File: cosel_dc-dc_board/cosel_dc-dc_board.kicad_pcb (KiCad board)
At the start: 2 copper layers, 105 x 80 mm, 15 parts, among them J1 B2PS-VH(LF)(SN), J2 Screw_Terminal_01x02, J3 Screw_Terminal_01x02, U1 CBS

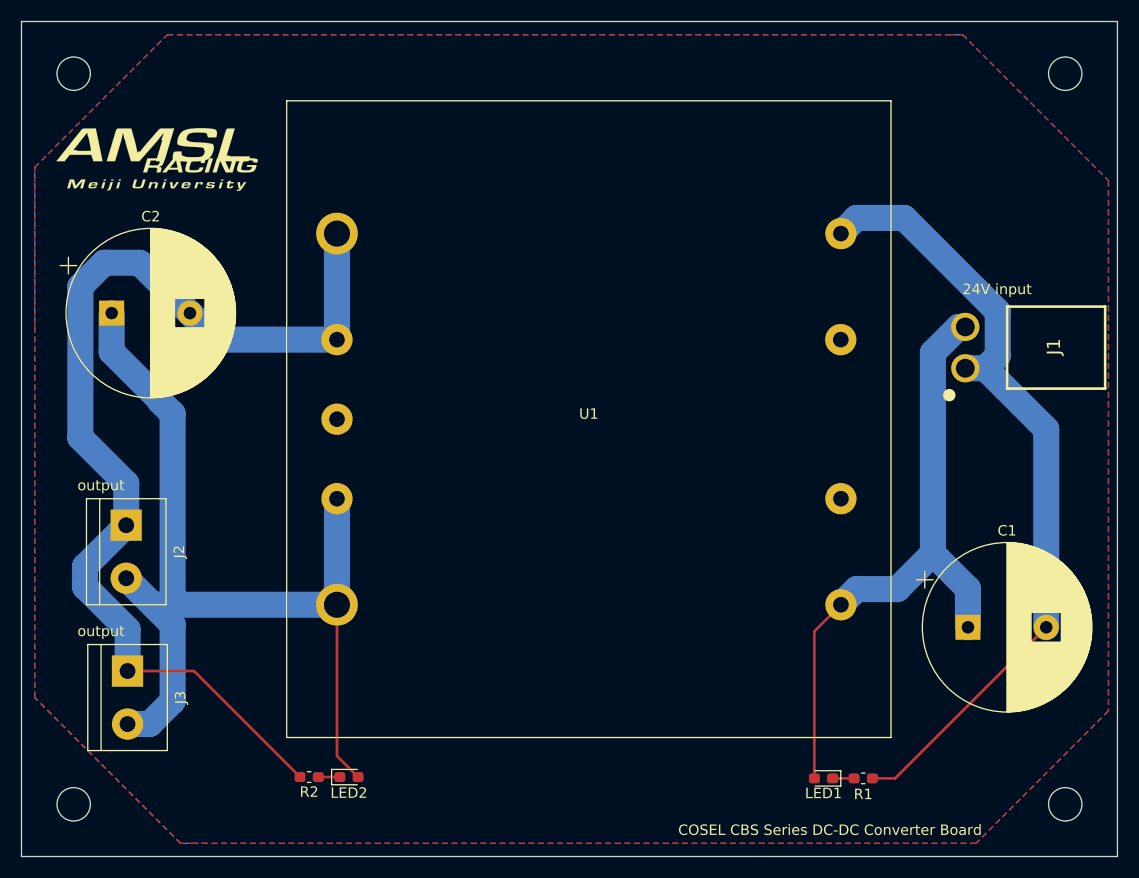
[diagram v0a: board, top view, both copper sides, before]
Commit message: update
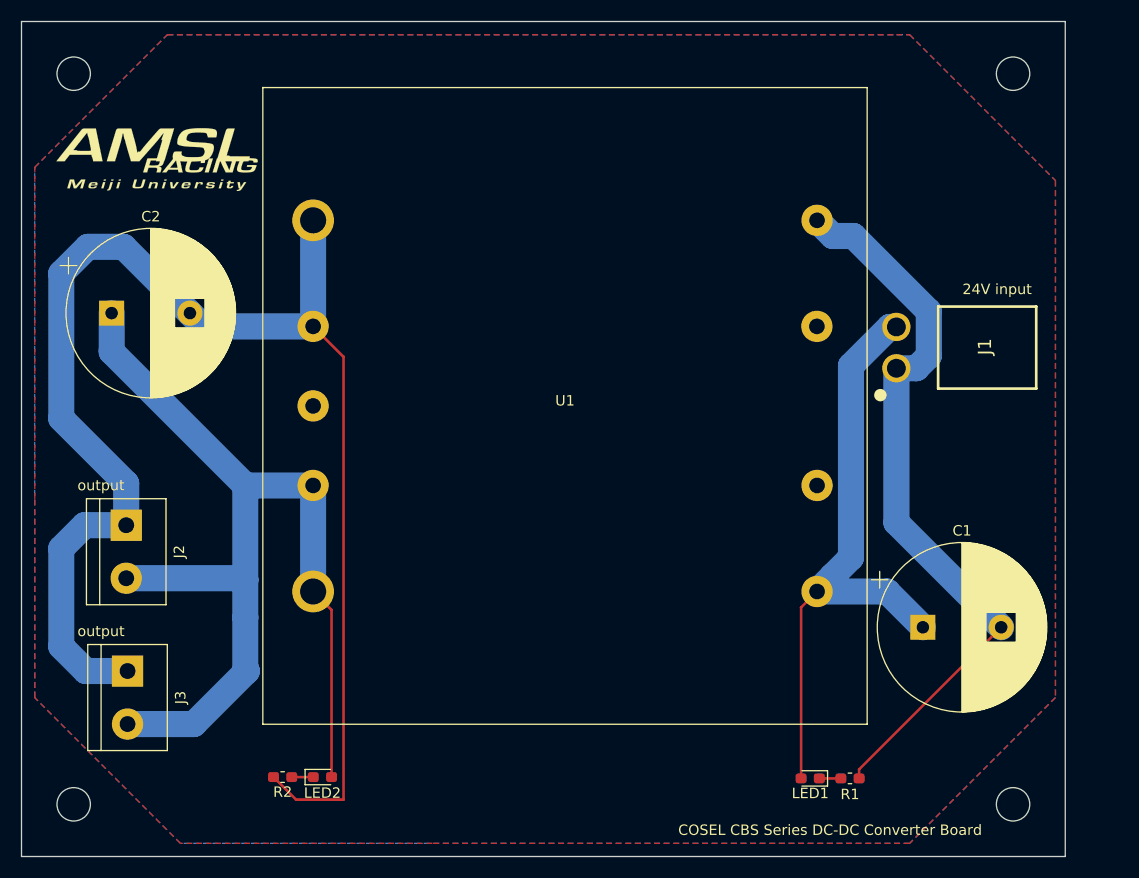
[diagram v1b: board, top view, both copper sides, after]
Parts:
- moved J1 6.60 mm to (83.8, 31.2)
- moved REF** 5.00 mm to (95.0, 75.0)
- moved REF** 5.00 mm to (95.0, 5.00)
- moved C1 4.32 mm to (86.4, 58.0)
- moved U1 2.62 mm to (52.1, 36.8)
- moved R2 2.54 mm to (25.0, 72.4)
- moved LED2 2.54 mm to (28.8, 72.4)
- moved LED1 1.27 mm to (75.6, 72.5)
- moved R1 1.27 mm to (79.4, 72.5)
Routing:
- net GNDPWR: track 101.5 -> 143.2 mm
- net GND: track 77.4 -> 71.3 mm
- net Net-(C2-Pad1): track 94.4 -> 99.8 mm
- net +24V: track 60.4 -> 59.0 mm
- added copper zone on B.Cu, net GND
- added copper zone on F.Cu, net GNDPWR
- removed copper zone on F.Cu, net GND
- removed copper zone on B.Cu, net GNDPWR
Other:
- board size 105 x 80 mm -> 100 x 80 mm
